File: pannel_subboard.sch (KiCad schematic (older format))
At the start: 12 parts, among them J1 Conn_01x02, J10 Conn_02x14_Counter_Clockwise, J2 Conn_01x05, J3 Conn_01x05, J4 Conn_01x05, J5 Conn_01x05, J6 Conn_01x05, J7 Conn_01x05, J8 Conn_01x05, J9 Conn_01x05

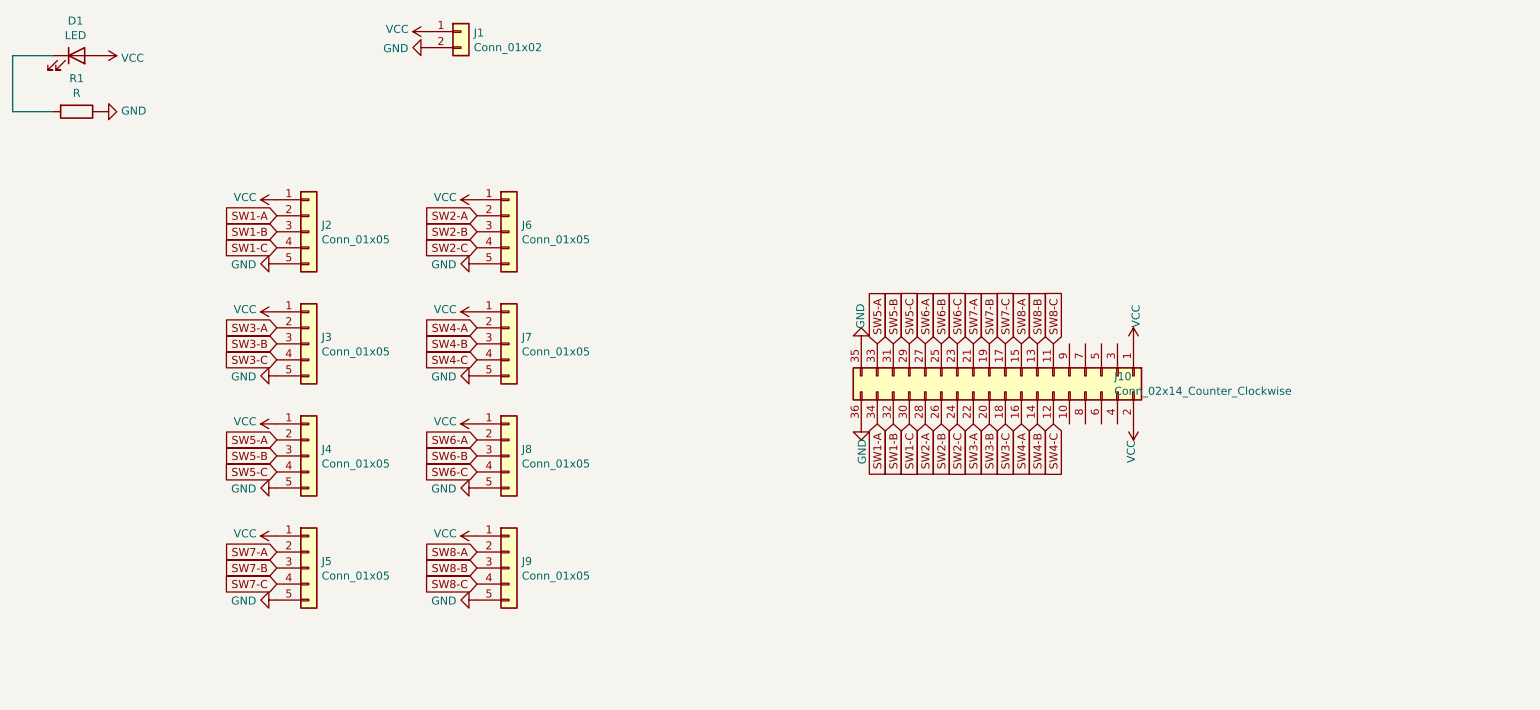
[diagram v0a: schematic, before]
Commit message: updates
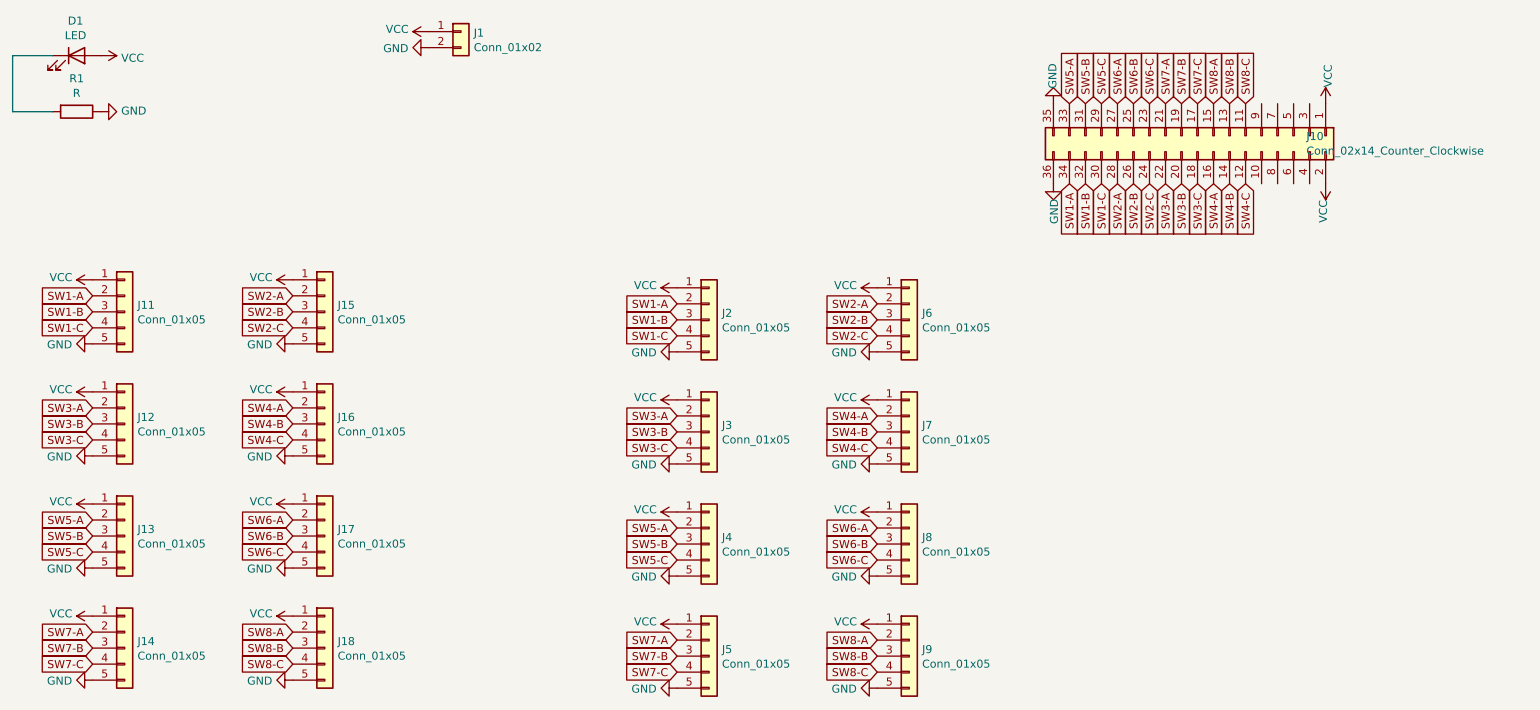
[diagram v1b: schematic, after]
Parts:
- added J11, J12, J13, J14, J15, J16, J17, J18: Conn_01x05, Pin_Headers:Pin_Header_Straight_1x05_Pitch2.54mm, symbol Connector_Generic:Conn_01x05
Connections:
- net GND: now also J11.5 (Pin_5), J12.5 (Pin_5), J13.5 (Pin_5), J14.5 (Pin_5), J15.5 (Pin_5), J16.5 (Pin_5), J17.5 (Pin_5), J18.5 (Pin_5)
- net SW1-A: now also J11.2 (Pin_2)
- net SW1-B: now also J11.3 (Pin_3)
- net SW1-C: now also J11.4 (Pin_4)
- net SW2-A: now also J15.2 (Pin_2)
- net SW2-B: now also J15.3 (Pin_3)
- net SW2-C: now also J15.4 (Pin_4)
- net SW3-A: now also J12.2 (Pin_2)
- net SW3-B: now also J12.3 (Pin_3)
- net SW3-C: now also J12.4 (Pin_4)
- net SW4-A: now also J16.2 (Pin_2)
- net SW4-B: now also J16.3 (Pin_3)
- net SW4-C: now also J16.4 (Pin_4)
- net SW5-A: now also J13.2 (Pin_2)
- net SW5-B: now also J13.3 (Pin_3)
- net SW5-C: now also J13.4 (Pin_4)
- net SW6-A: now also J17.2 (Pin_2)
- net SW6-B: now also J17.3 (Pin_3)
- net SW6-C: now also J17.4 (Pin_4)
- net SW7-A: now also J14.2 (Pin_2)
- net SW7-B: now also J14.3 (Pin_3)
- net SW7-C: now also J14.4 (Pin_4)
- net SW8-A: now also J18.2 (Pin_2)
- net SW8-B: now also J18.3 (Pin_3)
- net SW8-C: now also J18.4 (Pin_4)
- net VCC: now also J11.1 (Pin_1), J12.1 (Pin_1), J13.1 (Pin_1), J14.1 (Pin_1), J15.1 (Pin_1), J16.1 (Pin_1), J17.1 (Pin_1), J18.1 (Pin_1)
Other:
- moved on the sheet: J10, J2, J3, J4, J5, J6, J7, J8, J9
